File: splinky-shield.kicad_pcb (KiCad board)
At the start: 2 copper layers, 73.5 x 50.8 mm, 53 parts, among them J1 USB_C_Receptacle_USB2.0, J10 Ribbon, J2 Conn_01x04_Female, J3 Conn_01x04_Female, J5 Conn_01x02, J50 Conn_01x04_Female, J6 Serial, J7 trackball, J8 Ribbon, J9 RGB, SW3 SW_SPST, U1 RP2040, U2 GD25Q80CEIGR, U3 XC6210B332MR-G, Y1 Crystal_GND24

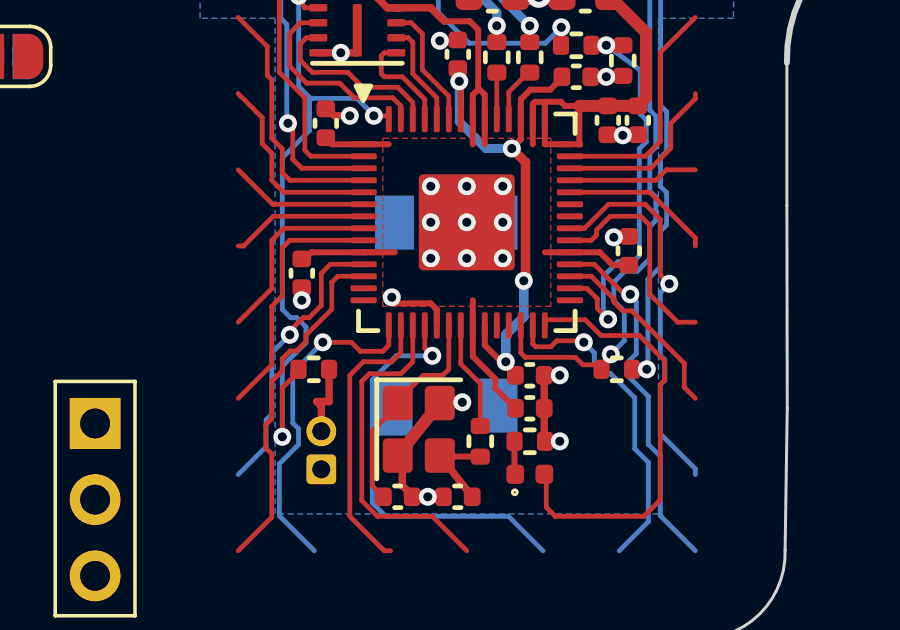
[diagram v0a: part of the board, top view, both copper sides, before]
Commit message: rst button both sides...
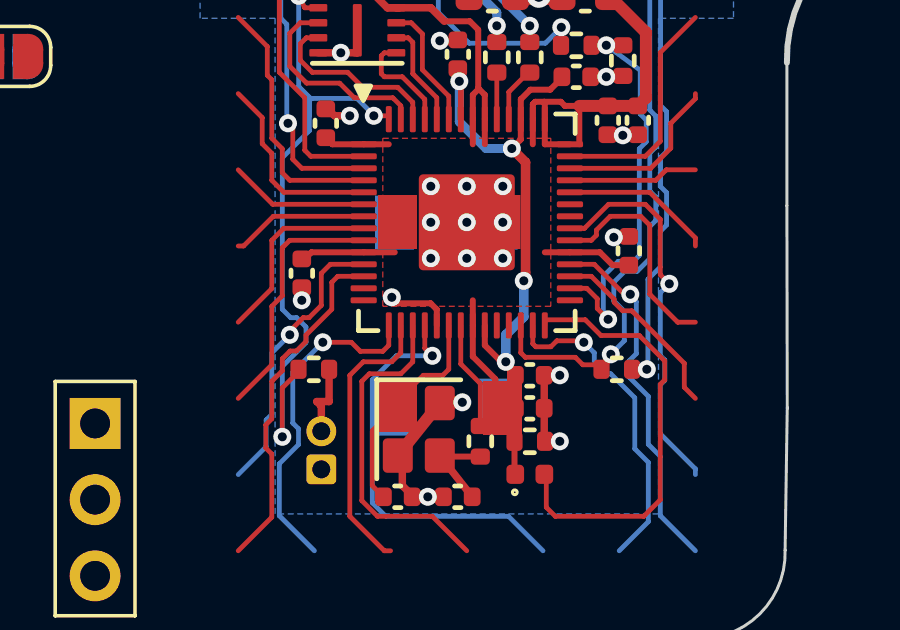
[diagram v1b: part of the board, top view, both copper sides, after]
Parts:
- added SW3: SW_SPST, Library:PushSwitch, F.Cu at (151.8, 100.1)
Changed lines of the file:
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@@
+    )
+  )
+  (footprint "Library:PushSwitch" (layer "F.Cu")
+    (at 151.79 100.09 -90)
+    (descr "tactile push button, 6x6mm e.g. PTS645xx series, height=9.5mm")
+    (tags "tact sw push 6mm smd")
+    (property "Sheetfile" "splinky-shield.kicad_sch")
+    (property "Sheetname" "")
+    (attr smd exclude_from_pos_files)
+    (fp_text reference "SW3" (at 0 -4 90) (layer "F.SilkS") hide
+      (effects (font (size 1 1) (thickness 0.15)))
+    )
+    (fp_text value "SW_SPST" (at 0 4.15 90) (layer "F.Fab")
+      (effects (font (size 1 1) (thickness 0.15)))
+    )
+    (fp_text user "${REFERENCE}" (at 0 -4 90) (layer "F.Fab")
+      (effects (font (size 1 1) (thickness 0.15)))
+    )
+    (fp_line (start -3 3) (end 3 3) (layer "F.Fab") (width 0.1))
+    (fp_line (start 3 -3) (end -3 -3) (layer "F.Fab") (width 0.1))
+    (fp_line (start 3 3) (end 3 -3) (layer "F.Fab") (width 0.1))
+    (fp_line (start -3 -3) (end -3 3) (layer "F.Fab") (width 0.1))
+    (fp_circle (center 0 0) (end 1 0) (layer "F.Fab") (width 0.1) (fill none))
+    (pad "1" smd rect (at 3.1 -1.8 270) (size 1.8 1.3) (layers "F.Cu" "F.Paste" "F.Mask")
+      (pinfunction "A") (pintype "passive"))
+    (pad "1" smd rect (at -3.1 -1.75 270) (size 1.8 1.3) (layers "F.Cu" "F.Paste" "F.Mask")
+      (pinfunction "A") (pintype "passive"))
+    (pad "2" smd rect (at -3.1 1.7 270) (size 1.8 1.3) (layers "F.Cu" "F.Paste" "F.Mask")
+      (pinfunction "B") (pintype "passive"))
+    (pad "2" smd rect (at 3 1.7 270) (size 1.8 1.3) (layers "F.Cu" "F.Paste" "F.Mask")
+      (pinfunction "B") (pintype "passive"))
+    (model "${KISYS3DMOD}/Button_Switch_SMD.3dshapes/SW_PUSH_6mm_H9.5mm.wrl"
+      (offset (xyz 0 0 0))
+      (scale (xyz 1 1 1))
+      (rotate (xyz 0 0 0))
     )
   )

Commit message: rst button :(
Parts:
- renumbered SW3 to SW1
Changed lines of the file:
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@@
     )
   )
-  (footprint "Library:PushSwitch" (layer "F.Cu")
+  (footprint "Library:PushSwitch" locked (layer "F.Cu")
     (at 151.79 100.09 -90)
     (descr "tactile push button, 6x6mm e.g. PTS645xx series, height=9.5mm")
@@
     (property "Sheetname" "")
     (attr smd exclude_from_pos_files)
-    (fp_text reference "SW3" (at 0 -4 90) (layer "F.SilkS") hide
+    (fp_text reference "SW1" (at 0 -4 90) (layer "F.SilkS") hide
       (effects (font (size 1 1) (thickness 0.15)))
     )
@@
     (fp_line (start -3 -3) (end -3 3) (layer "F.Fab") (width 0.1))
     (fp_circle (center 0 0) (end 1 0) (layer "F.Fab") (width 0.1) (fill none))
-    (pad "1" smd rect (at 3.1 -1.8 270) (size 1.8 1.3) (layers "F.Cu" "F.Paste" "F.Mask")
+    (pad "1" smd rect locked (at 3.1 -1.8 270) (size 1.8 1.3) (layers "F.Cu" "F.Paste" "F.Mask")
       (pinfunction "A") (pintype "passive"))
-    (pad "1" smd rect (at -3.1 -1.75 270) (size 1.8 1.3) (layers "F.Cu" "F.Paste" "F.Mask")
+    (pad "1" smd rect locked (at -3.1 -1.75 270) (size 1.8 1.3) (layers "F.Cu" "F.Paste" "F.Mask")
       (pinfunction "A") (pintype "passive"))
-    (pad "2" smd rect (at -3.1 1.7 270) (size 1.8 1.3) (layers "F.Cu" "F.Paste" "F.Mask")
+    (pad "2" smd rect locked (at -3.1 1.7 270) (size 1.8 1.3) (layers "F.Cu" "F.Paste" "F.Mask")
       (pinfunction "B") (pintype "passive"))
-    (pad "2" smd rect (at 3 1.7 270) (size 1.8 1.3) (layers "F.Cu" "F.Paste" "F.Mask")
+    (pad "2" smd rect locked (at 3 1.7 270) (size 1.8 1.3) (layers "F.Cu" "F.Paste" "F.Mask")
       (pinfunction "B") (pintype "passive"))
     (model "${KISYS3DMOD}/Button_Switch_SMD.3dshapes/SW_PUSH_6mm_H9.5mm.wrl"
@@
       ) (layer "B.SilkS") (width 0) (fill solid))
   )
-  (footprint "Library:PushSwitch" (layer "B.Cu")
+  (footprint "Library:PushSwitch" locked (layer "B.Cu")
     (at 151.74 100.11 -90)
     (descr "tactile push button, 6x6mm e.g. PTS645xx series, height=9.5mm")
@@
     (fp_line (start -3 3) (end -3 -3) (layer "B.Fab") (width 0.1))
     (fp_circle (center 0 0) (end 1 0) (layer "B.Fab") (width 0.1) (fill none))
-    (pad "1" smd rect (at 3.1 1.8 270) (size 1.8 1.3) (layers "B.Cu" "B.Paste" "B.Mask")
+    (pad "1" smd rect locked (at 3.1 1.8 270) (size 1.8 1.3) (layers "B.Cu" "B.Paste" "B.Mask")
       (net 38 "Rst") (pinfunction "A") (pintype "passive"))
-    (pad "1" smd rect (at -3.1 1.75 270) (size 1.8 1.3) (layers "B.Cu" "B.Paste" "B.Mask")
+    (pad "1" smd rect locked (at -3.1 1.75 270) (size 1.8 1.3) (layers "B.Cu" "B.Paste" "B.Mask")
       (net 38 "Rst") (pinfunction "A") (pintype "passive"))
-    (pad "2" smd rect (at -3.1 -1.7 270) (size 1.8 1.3) (layers "B.Cu" "B.Paste" "B.Mask")
+    (pad "2" smd rect locked (at -3.1 -1.7 270) (size 1.8 1.3) (layers "B.Cu" "B.Paste" "B.Mask")
       (net 2 "GND") (pinfunction "B") (pintype "passive"))
-    (pad "2" smd rect (at 3 -1.7 270) (size 1.8 1.3) (layers "B.Cu" "B.Paste" "B.Mask")
+    (pad "2" smd rect locked (at 3 -1.7 270) (size 1.8 1.3) (layers "B.Cu" "B.Paste" "B.Mask")
       (net 2 "GND") (pinfunction "B") (pintype "passive"))
     (model "${KISYS3DMOD}/Button_Switch_SMD.3dshapes/SW_PUSH_6mm_H9.5mm.wrl"
